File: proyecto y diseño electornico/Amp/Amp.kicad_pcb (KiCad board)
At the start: 2 copper layers, 60 x 36 mm, 24 parts, among them J1 Cable_PAD, J2 Cable_PAD, J3 Cable_PAD, J4 Cable_PAD, J5 Cable_PAD, J6 Cable_PAD, Q1 BC546, Q2 LND150, U1 TA8200AH

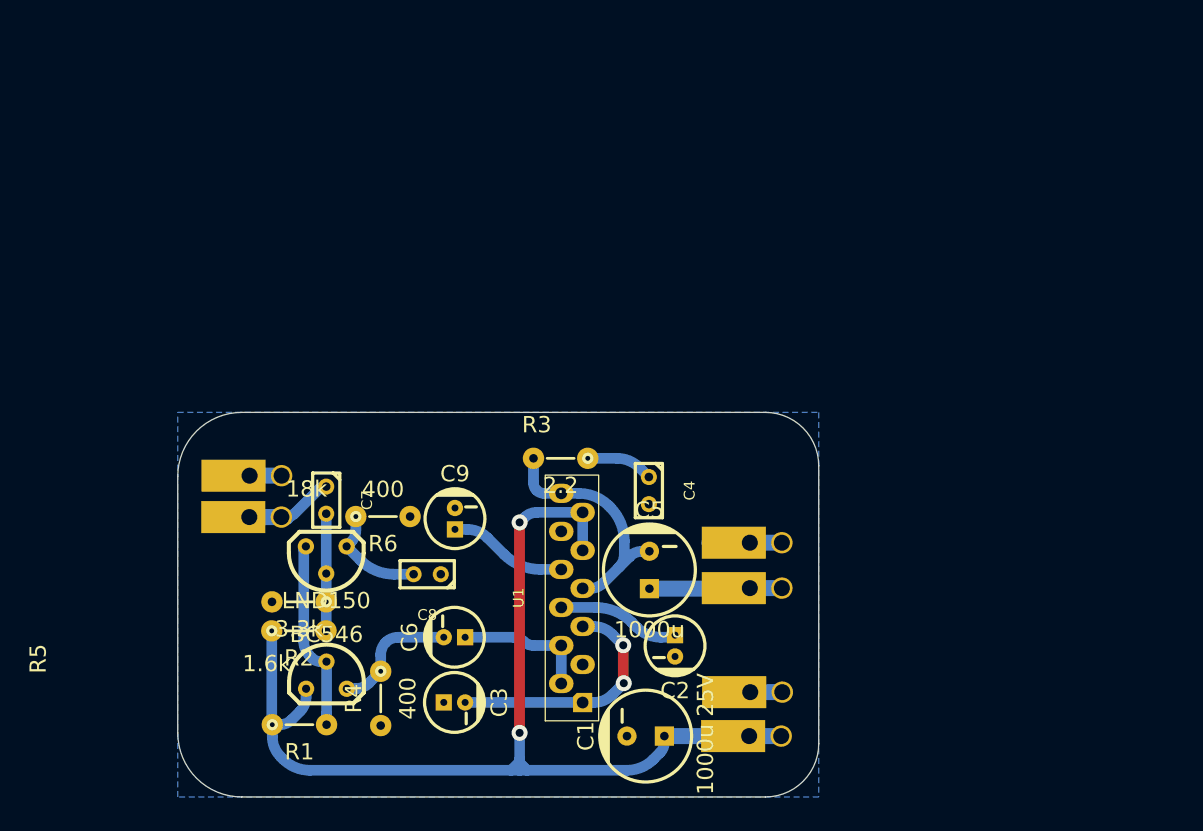
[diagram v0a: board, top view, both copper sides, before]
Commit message: 1/11
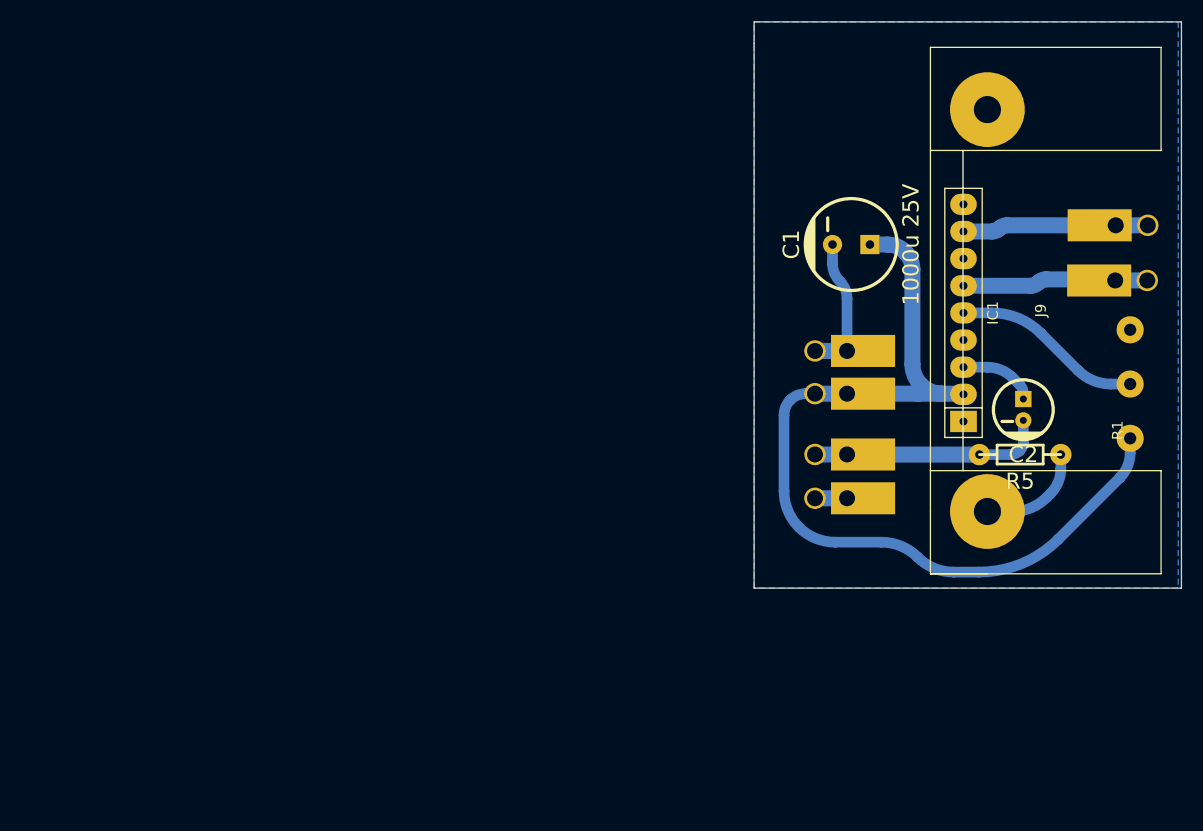
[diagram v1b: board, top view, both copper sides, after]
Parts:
- removed C3, C9: 47u, EESTN5:CAP_ELEC_5x11mm
- removed C4: 120n, EESTN5:CAP_0.1
- removed C5: 1000u, EESTN5:CAP_ELEC_8x11.5mm
- removed C6: 2.2u, EESTN5:CAP_ELEC_5x11mm
- removed C7: 470n/390n, EESTN5:CAP_0.1
- removed C8: 150n, EESTN5:CAP_0.1
- removed Q1: BC546, EESTN5:to92
- removed Q2: LND150, EESTN5:to92
- removed R2: 18k, EESTN5:RES0.2
- removed R3: 2.2, EESTN5:RES0.2
- removed R4, R6: 400, EESTN5:RES0.2
- removed U1: TA8200AH, MacroLib:hzip12-p-1.78
- added IC1: TDA7056A, MacroLib:SOT-110, F.Cu at (190.6, 74.2)
- added J9: DISIPADOR, MacroLib:Disipador_SOT110-1, F.Cu at (192.8, 74.0)
- C2: value 47u -> 0.47u
- R1: value 1.6k -> 10k; footprint EESTN5:RES0.2 -> EESTN5:Potenciometro
- R5: value 3.3k -> 5.1k; footprint EESTN5:RES0.2 -> EESTN5:RES0.3
- moved R1 84.0 mm to (206.2, 80.9), turned to -90 degrees
- moved R5 68.9 mm to (195.9, 87.5)
- moved J5 56.3 mm to (179.7, 87.5), turned to 90 degrees
- moved J6 56.0 mm to (179.7, 91.6), turned to 90 degrees
- moved C1 49.9 mm to (180.1, 67.8)
- moved J4 45.3 mm to (204.8, 66.0)
- moved J3 44.7 mm to (204.8, 71.2)
- moved C2 39.4 mm to (196.2, 83.3)
- moved J2 33.3 mm to (179.7, 81.8), turned to 90 degrees
- moved J1 33.2 mm to (179.7, 77.8), turned to 90 degrees
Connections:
- C2 pad 2: GND -> /amp_in
- J3 pad 1: /amp_out -> /amp_out+
- J4 pad 1: GND -> /amp_out-
- J5 pad 1: /pre_amp_in -> /amp_in
- R1 pad 1: VCC -> GND
- R1 pad 2: Net-(Q1-Pad2) -> /Vcontrol
- R5 pad 1: Net-(C7-Pad2) -> GND
- R5 pad 2: GND -> /amp_in
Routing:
- net Net-(C5-Pad2): track 24.9 -> 0.00 mm
- net Net-(C3-Pad2): track 23.5 -> 0.00 mm, vias 2 -> 0
- net /amp_in: track 0.00 -> 22.2 mm
- net Net-(Q1-Pad2): track 18.1 -> 0.00 mm
- net /Vcontrol: track 0.00 -> 17.8 mm
- net /amp_out-: track 0.00 -> 17.4 mm
- net /amp_out+: track 0.00 -> 14.6 mm
- net GND: track 13.0 -> 26.6 mm
- net VCC: track 102.0 -> 88.8 mm, vias 2 -> 0
- net /out_pre_amp: track 12.8 -> 0.00 mm
- net /amp_out: track 12.4 -> 0.00 mm
- net Net-(C6-Pad2): track 12.1 -> 0.00 mm
- net Net-(C9-Pad1): track 11.1 -> 0.00 mm
- net Net-(C7-Pad2): track 11.0 -> 0.00 mm
- net Net-(C8-Pad2): track 10.1 -> 0.00 mm
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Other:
- board size 60 x 36 mm -> 40 x 53 mm
